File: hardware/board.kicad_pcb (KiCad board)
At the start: 2 copper layers, 146 x 40 mm, 65 parts, among them IC1 DW01A, J1 Conn_01x03_Male, J2 Conn_01x03_Male, J3 Conn_01x06, J4 Conn_01x06_Female, J5 Conn_01x06, J6 Conn_01x04, J7 Conn_01x02, P1 USB_C_Plug_USB2.0, Q1 AO3400A, Q2 AO3400A, Q3 AO3401A, Q4 FS8205A, SW1 SW_Push, SW2 SW_Push, SW3 SW_SPST, U1 HT7850-1-SOT89, U2 HT7833-1-SOT89, U3 ESP32-WROOM-32, U4 MPU-6050, U5 MT3608, U6 TP4056

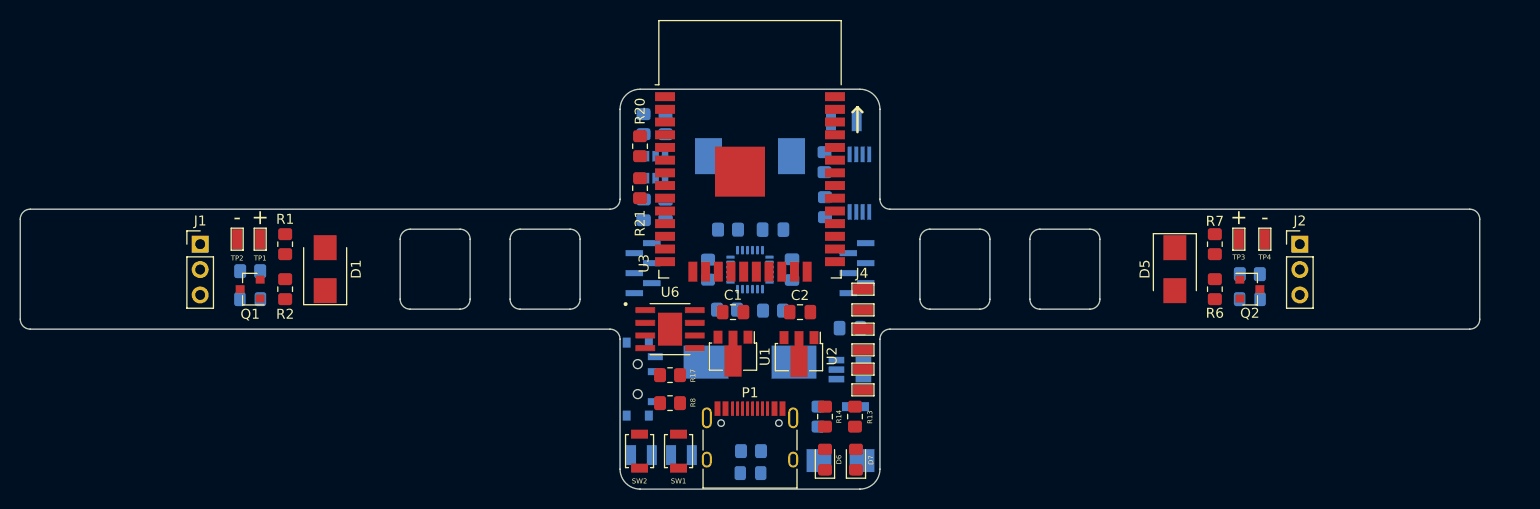
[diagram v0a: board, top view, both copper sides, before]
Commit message: PCB routed
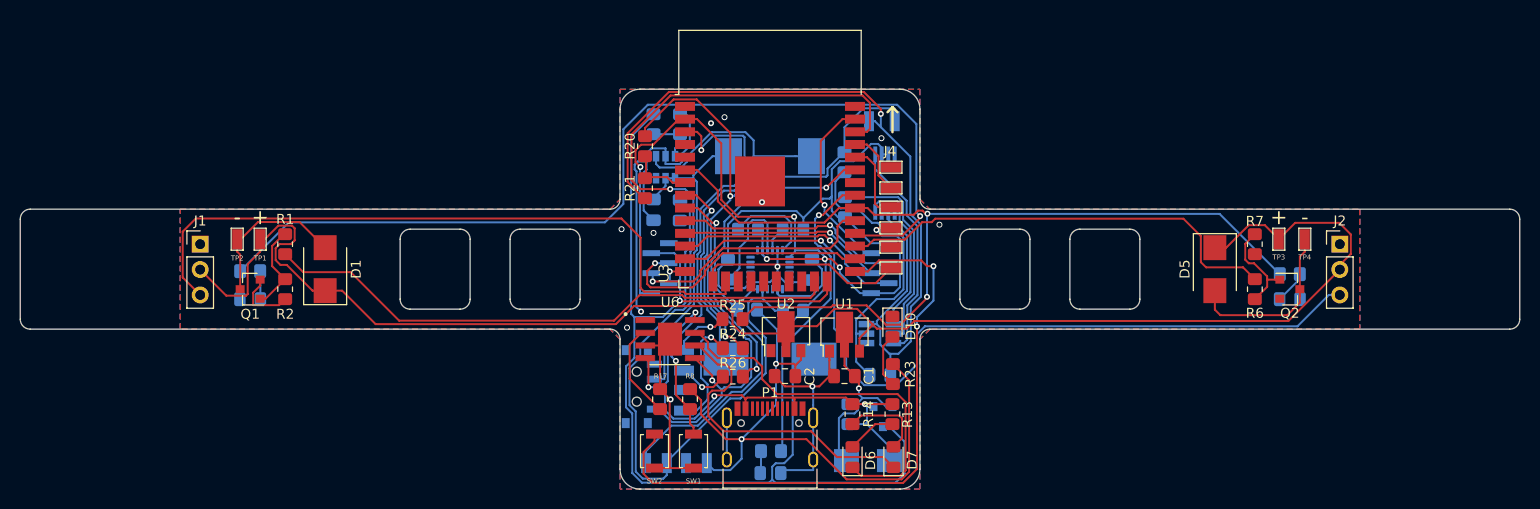
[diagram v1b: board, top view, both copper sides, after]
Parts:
- added D10: LED, LED_SMD:LED_0805_2012Metric_Pad1.15x1.40mm_HandSolder, F.Cu at (171.2, 82.8)
- added J8: Conn_01x04, Board:Wire-Pad-01x04, B.Cu at (150.5, 90.8)
- added R23: 1k, Resistor_SMD:R_0805_2012Metric_Pad1.20x1.40mm_HandSolder, F.Cu at (171.3, 87.5)
- added R24: 100R, Resistor_SMD:R_0805_2012Metric_Pad1.20x1.40mm_HandSolder, F.Cu at (155.3, 84.9)
- added R25: 1k, Resistor_SMD:R_0805_2012Metric_Pad1.20x1.40mm_HandSolder, F.Cu at (155.2, 82.0)
- added R26: 1k, Resistor_SMD:R_0805_2012Metric_Pad1.20x1.40mm_HandSolder, F.Cu at (155.3, 87.8)
- SW3: footprint Button_Switch_SMD:SW_SPDT_PCM12 -> Board:SW_SPDT_PCM12
- moved C1 12.9 mm to (166.4, 87.7), turned to 180 degrees
- moved J4 12.5 mm to (171.0, 67.2)
- moved U1 11.3 mm to (166.4, 83.5), turned to 90 degrees
- moved C2 6.57 mm to (160.5, 87.7), turned to 180 degrees
- moved C7 5.58 mm to (170.0, 87.6), turned to 0 degrees
- moved IC1 4.69 mm to (170.0, 83.5), turned to 180 degrees
- moved D4 4.00 mm to (211.0, 80.0)
- moved D5 4.00 mm to (203.5, 77.0)
- moved J2 4.00 mm to (216.0, 74.5)
- moved Q2 4.00 mm to (211.0, 79.0)
- moved R5 4.00 mm to (211.0, 77.5)
- moved R6 4.00 mm to (207.5, 79.0)
- moved R7 4.00 mm to (207.5, 74.5)
- moved TP3 4.00 mm to (209.9, 77.0)
- moved TP4 4.00 mm to (212.5, 77.0)
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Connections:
- net /Sheet623EC3BA/AD0 renamed Net-(R10-Pad1)
- net /Sheet623EC3BA/INT renamed Net-(R12-Pad2)
- J5 pad 2: /IO34 -> /IO27
- J5 pad 3: /IO33 -> /IO26
- J5 pad 4: /IO32 -> /IO25
- J5 pad 5: /IO27 -> /IO23
- U3 pad 10: (no net) -> /IO25
- U3 pad 11: (no net) -> /IO26
- U3 pad 37: (no net) -> /IO23
- U3 pad 6: /IO34 -> /LED_B
- U3 pad 8: /IO32 -> /LED_R
- U3 pad 9: /IO33 -> /LED_G
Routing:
- net +5V: track 0.00 -> 165.1 mm
- net GND: track 0.00 -> 162.4 mm, vias 0 -> 12
- net +3V3: track 0.00 -> 150.3 mm, vias 0 -> 8
- net /SCL: track 0.00 -> 104.2 mm, vias 0 -> 1
- net /Sheet6241753E/BATT+_OUT: track 0.00 -> 102.7 mm
- net /LED_A: track 0.00 -> 96.6 mm, vias 0 -> 1
- net /LED_B: track 0.00 -> 95.2 mm, vias 0 -> 2
- net /Sheet6241753E/BATT-: track 0.00 -> 85.2 mm, vias 0 -> 1
- net /SERVO_B: track 0.00 -> 83.7 mm, vias 0 -> 1
- net /Sheet6241753E/BATT+: track 0.00 -> 79.2 mm, vias 0 -> 2
- net /SERVO_A: track 0.00 -> 69.2 mm
- net /IO0: track 0.00 -> 62.3 mm, vias 0 -> 2
- net /MOTOR_A: track 0.00 -> 58.3 mm
- net /Sheet6241753E/VBUS: track 0.00 -> 53.3 mm, vias 0 -> 4
- net /SDA: track 0.00 -> 51.6 mm, vias 0 -> 1
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- added copper zone on B.Cu, net GND
- added copper zone on F.Cu, net GND
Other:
- board size 146 x 40 mm -> 150 x 40 mm
- net class Default: clearance 0.2 -> 0.15; via_dia 0.8 -> 0.6
- rule trace_clearance: 0.2 -> 0.15
